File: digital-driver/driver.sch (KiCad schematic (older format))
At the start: 14 parts, among them J1 LDD-1500L, J2 Conn_01x02, J3 Barrel_Jack, J4 Conn_01x04, J5 Conn_01x04, J6 Barrel_Jack, J7 Conn_01x04, U1 ATtiny85-20PU

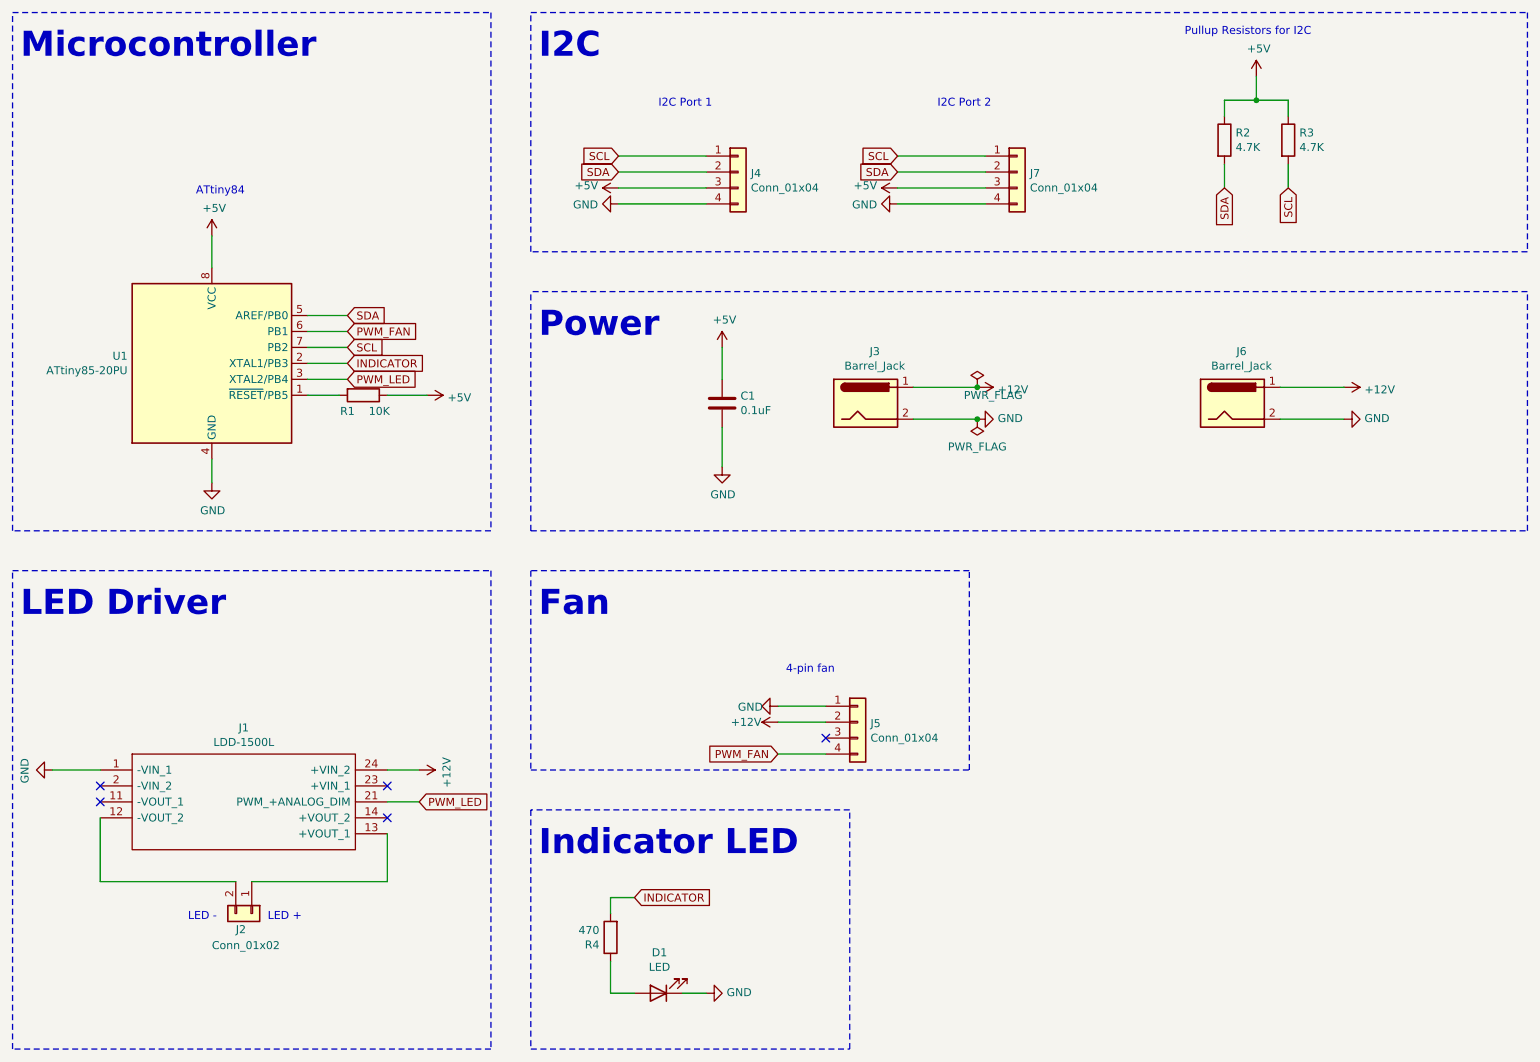
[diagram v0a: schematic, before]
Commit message: digital driver prototype
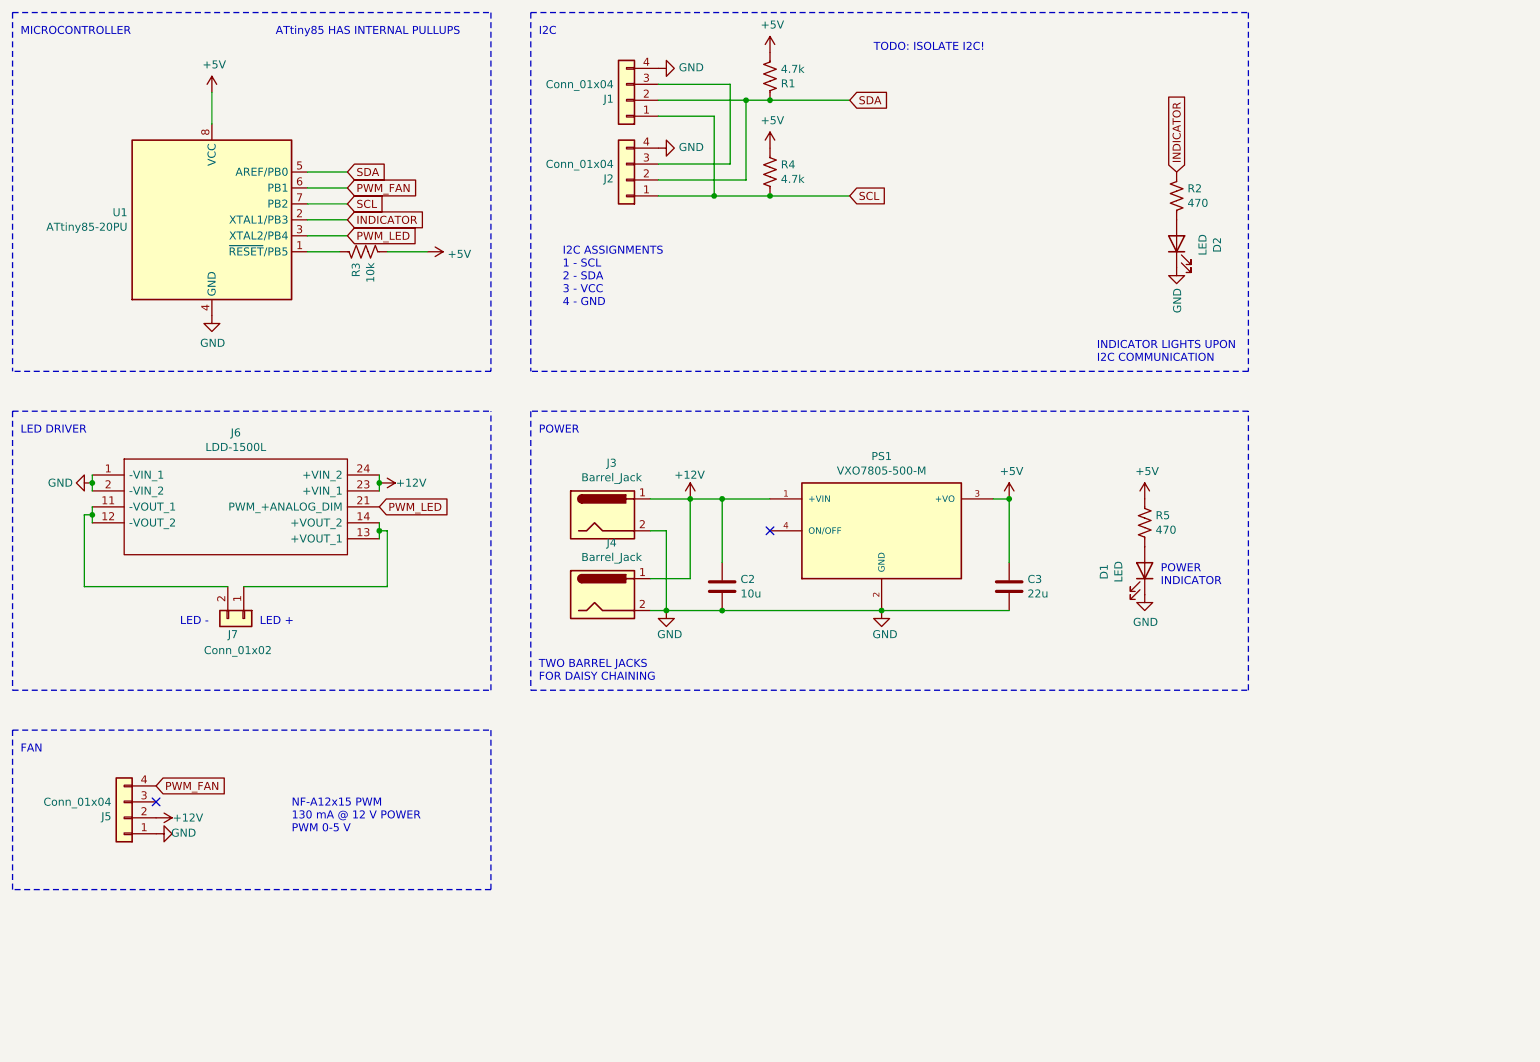
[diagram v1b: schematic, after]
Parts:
- removed C1: 0.1uF, Capacitor_SMD:C_1206_3216Metric, symbol Device:C
- removed R1: 10K, Resistor_SMD:R_1206_3216Metric, symbol Device:R
- removed R2, R3: 4.7K, Resistor_SMD:R_1206_3216Metric, symbol Device:R
- removed R4: 470, Resistor_SMD:R_1206_3216Metric, symbol Device:R
- added C2: 10u, Capacitor_SMD:C_1206_3216Metric_Pad1.33x1.80mm_HandSolder, symbol Device:C
- added C3: 22u, Capacitor_SMD:C_1206_3216Metric_Pad1.33x1.80mm_HandSolder, symbol Device:C
- added D1: LED, LED_SMD:LED_1206_3216Metric, symbol Device:LED
- added PS1: VXO7805-500-M, CONV_VXO7805-500-M, symbol VXO7805-500-M:VXO7805-500-M
- added R1, R4: 4.7k, Resistor_SMD:R_1206_3216Metric_Pad1.30x1.75mm_HandSolder, symbol Device:R_US
- added R2, R5: 470, Resistor_SMD:R_1206_3216Metric_Pad1.30x1.75mm_HandSolder, symbol Device:R_US
- added R3: 10k, Resistor_SMD:R_1206_3216Metric_Pad1.30x1.75mm_HandSolder, symbol Device:R_US
- renumbered D1 to D2, J4 to J1, J7 to J2, J6 to J4, J1 to J6, J2 to J7
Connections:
- net +12V: now also J6.23 (+VIN_1), C2.2, PS1.1 (+VIN)
- net +5V: now also C3.1, PS1.3 (+VO), R1.2, R3.1, R4.1, R5.1; no longer J1.3 (Pin_3), J2.3 (Pin_3)
- net GND: now also J6.2 (-VIN_2), C2.1, C3.2, D1.1 (K), PS1.2 (GND)
- net INDICATOR: now also R2.1
- net SCL: now also R4.2
- net SDA: now also R1.1
- net at J6.13 (+VOUT_1), J7.1 (Pin_1): now also J6.14 (+VOUT_2)
- net at J6.12 (-VOUT_2), J7.2 (Pin_2): now also J6.11 (-VOUT_1)
- net at U1.1 (~RESET~/PB5): now also R3.2
- net at D2.2 (A): now also R2.2
- new net: J1.3 (Pin_3), J2.3 (Pin_3)
- new net: D1.2 (A), R5.2
- no-connect marks 5 -> 2
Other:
- note added: "ATtiny85 HAS INTERNAL PULLUPS"
- note added: "FAN"
- note added: "I2C ASSIGNMENTS\n1 - SCL\n2 - SDA\n3 - VCC\n4 - GND"
- note added: "INDICATOR LIGHTS UPON\nI2C COMMUNICATION"
- note added: "LED DRIVER"
- note added: "MICROCONTROLLER"
- note added: "NF-A12x15 PWM\n130 mA @ 12 V POWER\nPWM 0-5 V"
- note added: "POWER"
- note added: "POWER\nINDICATOR"
- note added: "TODO: ISOLATE I2C!"
- note added: "TWO BARREL JACKS\nFOR DAISY CHAINING"
- note removed: "4-pin fan"
- note removed: "ATtiny84"
- note removed: "Fan"
- note removed: "I2C Port 1"
- note removed: "I2C Port 2"
- note removed: "Indicator LED"
- note removed: "LED Driver"
- note removed: "Microcontroller"
- note removed: "Power"
- note removed: "Pullup Resistors for I2C"
- moved on the sheet: D2, J1, J2, J3, J4, J5, J6, J7, U1
